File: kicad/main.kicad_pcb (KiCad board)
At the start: 2 copper layers, 15 parts, among them J1 Barrel_Jack, J2 Conn, J3 VIA1, J4 VIA2, U1 DS1813-5+, U2 W65C816SxP, U3 L7805, U4 ATF16V8, U5 AS6C4008-55PCN, U6 27C512, U7 74LS573, U8 W65C22NxP, U9 74HC245, X1 CXO_DIP14

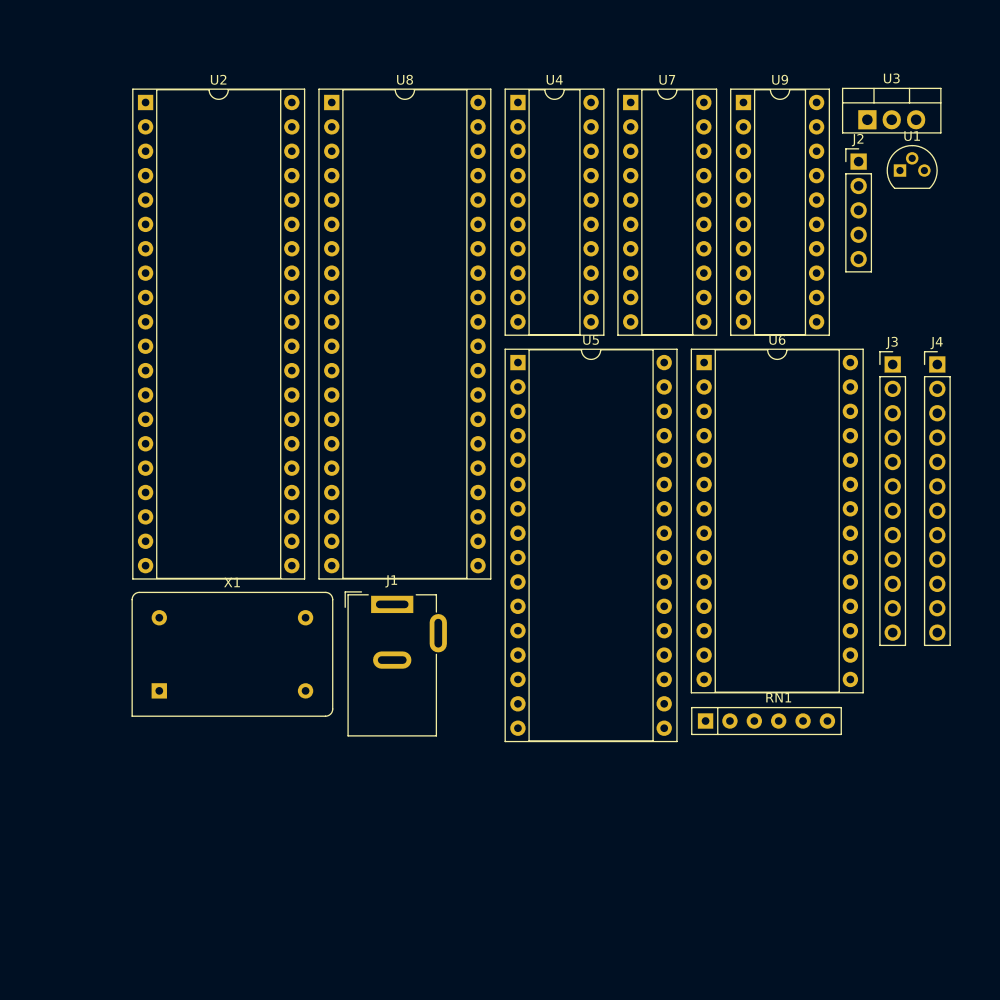
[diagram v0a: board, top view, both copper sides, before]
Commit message: v0.1 PCB
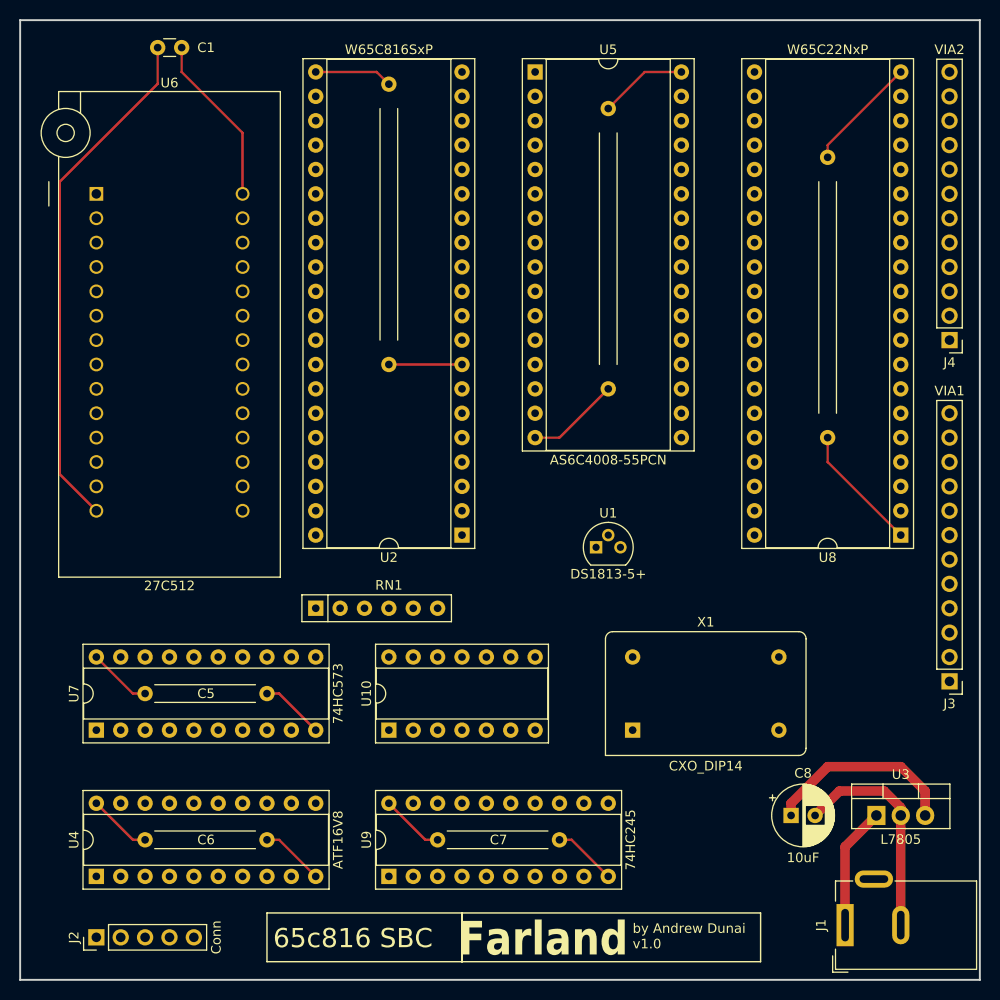
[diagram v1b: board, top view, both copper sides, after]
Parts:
- added C1: 0.1uF, Capacitor_THT:C_Disc_D3.0mm_W1.6mm_P2.50mm, F.Cu at (36.8, 22.9)
- added C2: 0.1uF, my:C_Disc_VeryLong, F.Cu at (58.4, 49.5)
- added C3: 0.1uF, my:C_Disc_VeryLong, F.Cu at (81.3, 35.6)
- added C4: 0.1uF, my:C_Disc_VeryLong, F.Cu at (104.1, 40.6)
- added C5: 0.1uF, my:C_Disc_Long, F.Cu at (33.0, 90.2)
- added C6: 0.1uF, my:C_Disc_Long, F.Cu at (33.0, 105.4)
- added C7: 0.1uF, my:C_Disc_Long, F.Cu at (63.5, 105.4)
- added C8: 10uF, Capacitor_THT:CP_Radial_D6.3mm_P2.50mm, F.Cu at (100.3, 102.9)
- added U10: 74HC14, Package_DIP:DIP-14_W7.62mm_Socket, F.Cu at (58.4, 94.0)
- U6: footprint Package_DIP:DIP-28_W15.24mm_Socket -> my:ZIF28
- U7: value 74LS573 -> 74HC573
- moved J2 113.3 mm to (27.9, 115.6), turned to 90 degrees
- moved U4 91.8 mm to (27.9, 109.2), turned to 90 degrees
- moved U9 88.7 mm to (58.4, 109.2), turned to 90 degrees
- moved U7 85.9 mm to (27.9, 94.0), turned to 90 degrees
- moved U8 74.5 mm to (111.8, 73.7), turned to 180 degrees
- moved U3 72.5 mm to (109.2, 102.9)
- moved U6 65.7 mm to (27.9, 38.1)
- moved J1 57.8 mm to (106.0, 114.3), turned to 90 degrees
- moved U2 55.9 mm to (66.0, 73.7), turned to 180 degrees
- moved U1 50.4 mm to (80.0, 74.9)
- moved X1 49.5 mm to (83.8, 94.0)
- moved RN1 42.3 mm to (50.8, 81.3)
- moved J3 33.5 mm to (116.8, 88.9), turned to 180 degrees
- moved U5 30.3 mm to (73.7, 25.4)
- moved J4 2.84 mm to (116.8, 53.3), turned to 180 degrees
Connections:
- U2 pad 39: unconnected-(U2-VDA-Pad39) -> VDA
- U4 pad 13: ~{CLK} -> Net-(U4-IO7)
- U4 pad 14: CLK -> Net-(U4-IO6)
- U8 pad 24: +5V -> VDA
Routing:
- net GND: track 0.00 -> 128.2 mm
- net +5V: track 0.00 -> 87.1 mm
- net Net-(U3-IN): track 0.00 -> 12.8 mm
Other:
- board outline added: 100 x 100 mm
- board text added: "65c816 SBC"
- board text added: "Farland"
- board text added: "by Andrew Dunai v1.0"

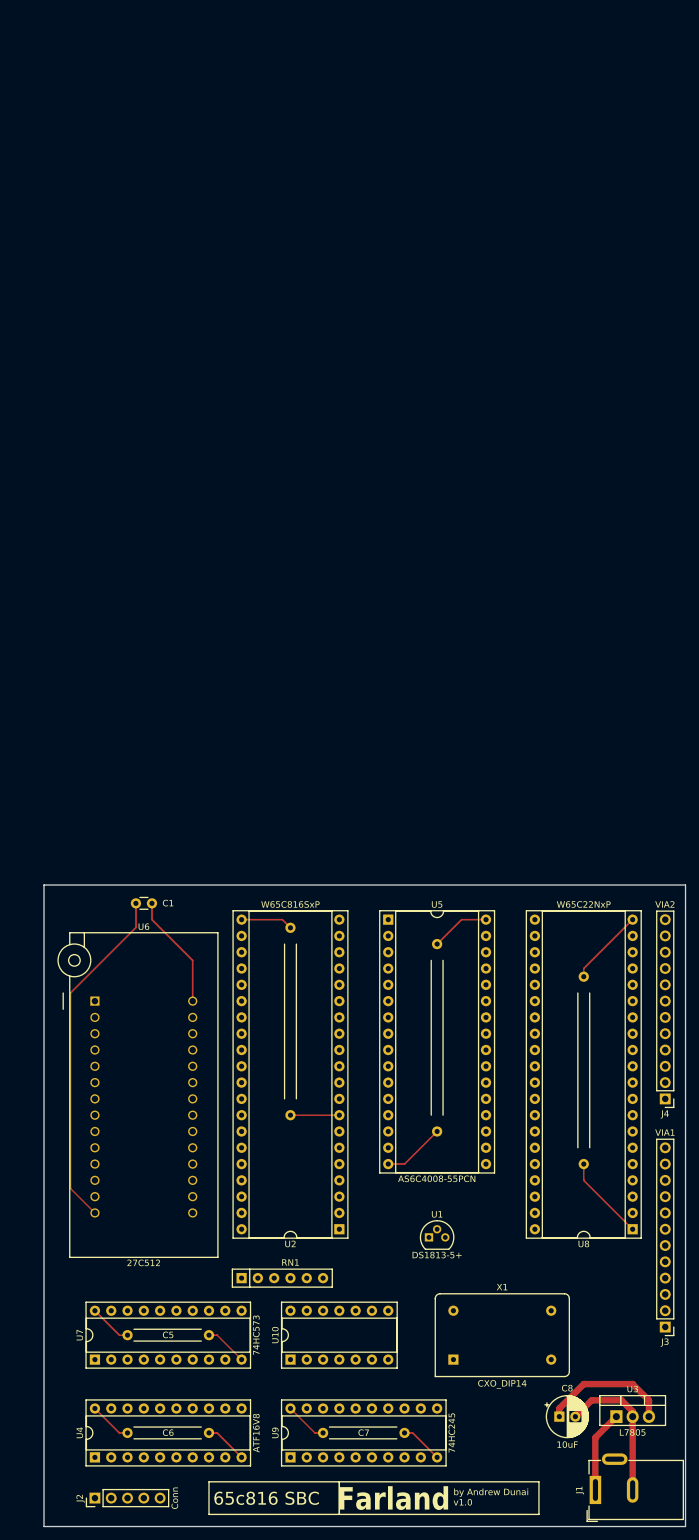
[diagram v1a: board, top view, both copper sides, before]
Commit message: v0.1 final PCB
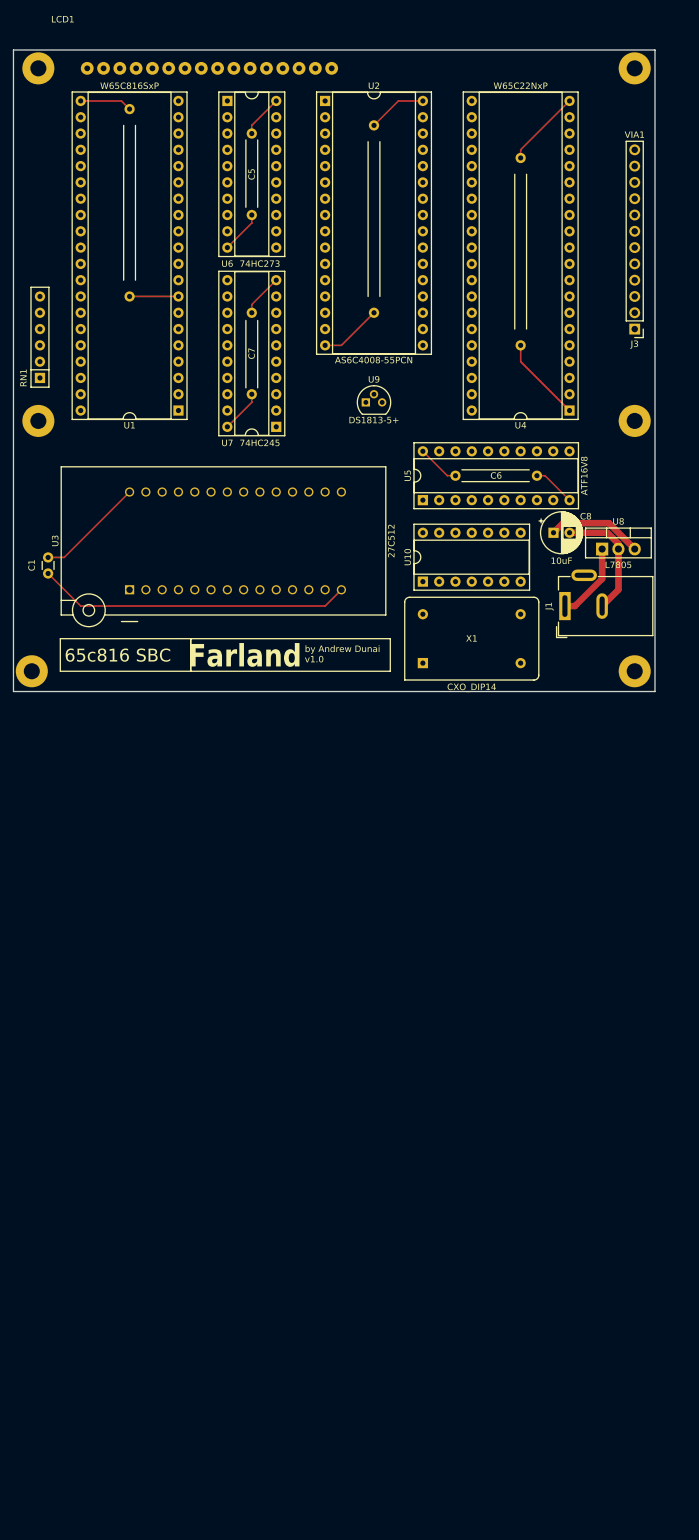
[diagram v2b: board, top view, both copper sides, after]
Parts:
- removed J2: Conn, Connector_PinHeader_2.54mm:PinHeader_1x05_P2.54mm_Vertical
- removed J4: VIA2, Connector_PinHeader_2.54mm:PinHeader_1x12_P2.54mm_Vertical
- removed the U7 at (27.9, 94.0)
- added H1: MountingHole_Pad, MountingHole:MountingHole_2.5mm_Pad, F.Cu at (18.1, -13.3)
- added H2: MountingHole_Pad, MountingHole:MountingHole_2.5mm_Pad, F.Cu at (112.1, -13.3)
- added LCD1: ~, my:2004A-OLED, F.Cu at (16.6, -109.8)
- added U6: 74HC273, Package_DIP:DIP-20_W7.62mm_Socket, F.Cu at (48.6, -102.2)
- moved C5 188.3 mm to (52.4, -97.1), turned to -90 degrees
- moved C7 162.3 mm to (52.4, -56.5), turned to 90 degrees
- moved U7 160.7 mm to (56.2, -51.4), turned to 180 degrees
- moved C6 157.7 mm to (84.1, -43.8)
- moved U5 157.7 mm to (79.1, -40.0)
- moved J3 155.6 mm to (112.1, -66.7)
- moved RN1 143.8 mm to (19.4, -59.0), turned to 90 degrees
- moved J1 137.9 mm to (101.2, -23.5)
- moved C8 137.8 mm to (99.4, -34.9)
- moved U8 135.3 mm to (107.0, -32.4)
- moved U9 130.5 mm to (70.2, -55.2)
- moved C2 130.1 mm to (33.3, -78.1)
- moved U1 130.1 mm to (41.0, -54.0)
- moved C3 128.0 mm to (71.4, -92.1)
- moved C4 128.0 mm to (94.3, -87.0)
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- renumbered U2 to U1, U5 to U2, U6 to U3, U8 to U4, U4 to U5, U9 to U7, U3 to U8, U1 to U9
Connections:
- U10 pad 1: Net-(U4-IO6) -> Net-(U5-IO7)
- U10 pad 3: Net-(U4-IO7) -> Net-(U5-IO8)
- U4 pad 10: Net-(J4-Pin_3) -> unconnected-(U4-PB0-Pad10)
- U4 pad 11: Net-(J4-Pin_4) -> unconnected-(U4-PB1-Pad11)
- U4 pad 12: Net-(J4-Pin_5) -> unconnected-(U4-PB2-Pad12)
- U4 pad 13: Net-(J4-Pin_6) -> unconnected-(U4-PB3-Pad13)
- U4 pad 14: Net-(J4-Pin_7) -> unconnected-(U4-PB4-Pad14)
- U4 pad 15: Net-(J4-Pin_8) -> unconnected-(U4-PB5-Pad15)
- U4 pad 16: Net-(J4-Pin_9) -> unconnected-(U4-PB6-Pad16)
- U4 pad 17: Net-(J4-Pin_10) -> unconnected-(U4-PB7-Pad17)
- U4 pad 18: Net-(J4-Pin_11) -> unconnected-(U4-CB1-Pad18)
- U4 pad 19: Net-(J4-Pin_12) -> unconnected-(U4-CB2-Pad19)
- U5 pad 12: unconnected-(U4-IO8-Pad12) -> Net-(U5-IO8)
- U5 pad 13: Net-(U4-IO7) -> Net-(U5-IO7)
- U5 pad 14: Net-(U4-IO6) -> ~{WD}
- U5 pad 15: ~{WD} -> ~{RD}
- U5 pad 16: ~{RD} -> LCDEN
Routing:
- net GND: track 128.2 -> 119.1 mm
- net +5V: track 87.1 -> 80.7 mm
- net Net-(U8-IN): track 12.8 -> 12.2 mm
